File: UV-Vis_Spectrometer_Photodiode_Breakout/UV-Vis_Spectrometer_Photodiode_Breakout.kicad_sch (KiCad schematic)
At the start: 32 parts, among them J1 Conn_01x05, J2 Conn_01x02, J3 Conn_01x02, Q1 NMOS, Q2 NMOS, Q3 NMOS, U1 TLV8811DBVR, U3 LTC2451

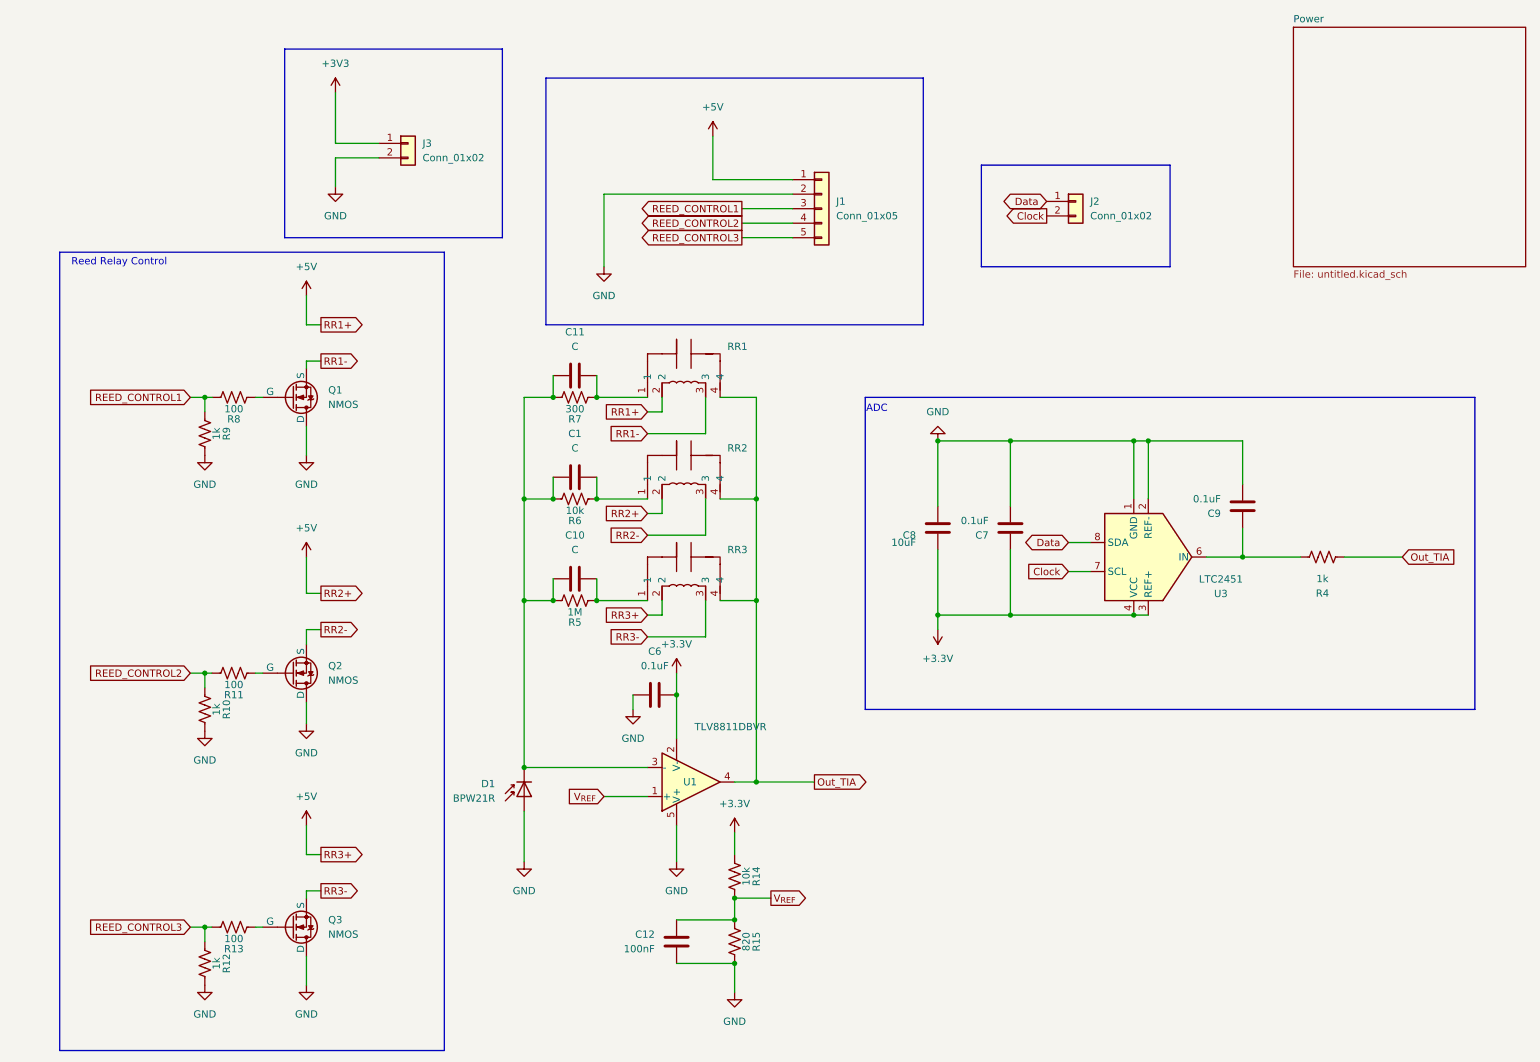
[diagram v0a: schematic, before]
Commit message: Made some nice boxes and labels.
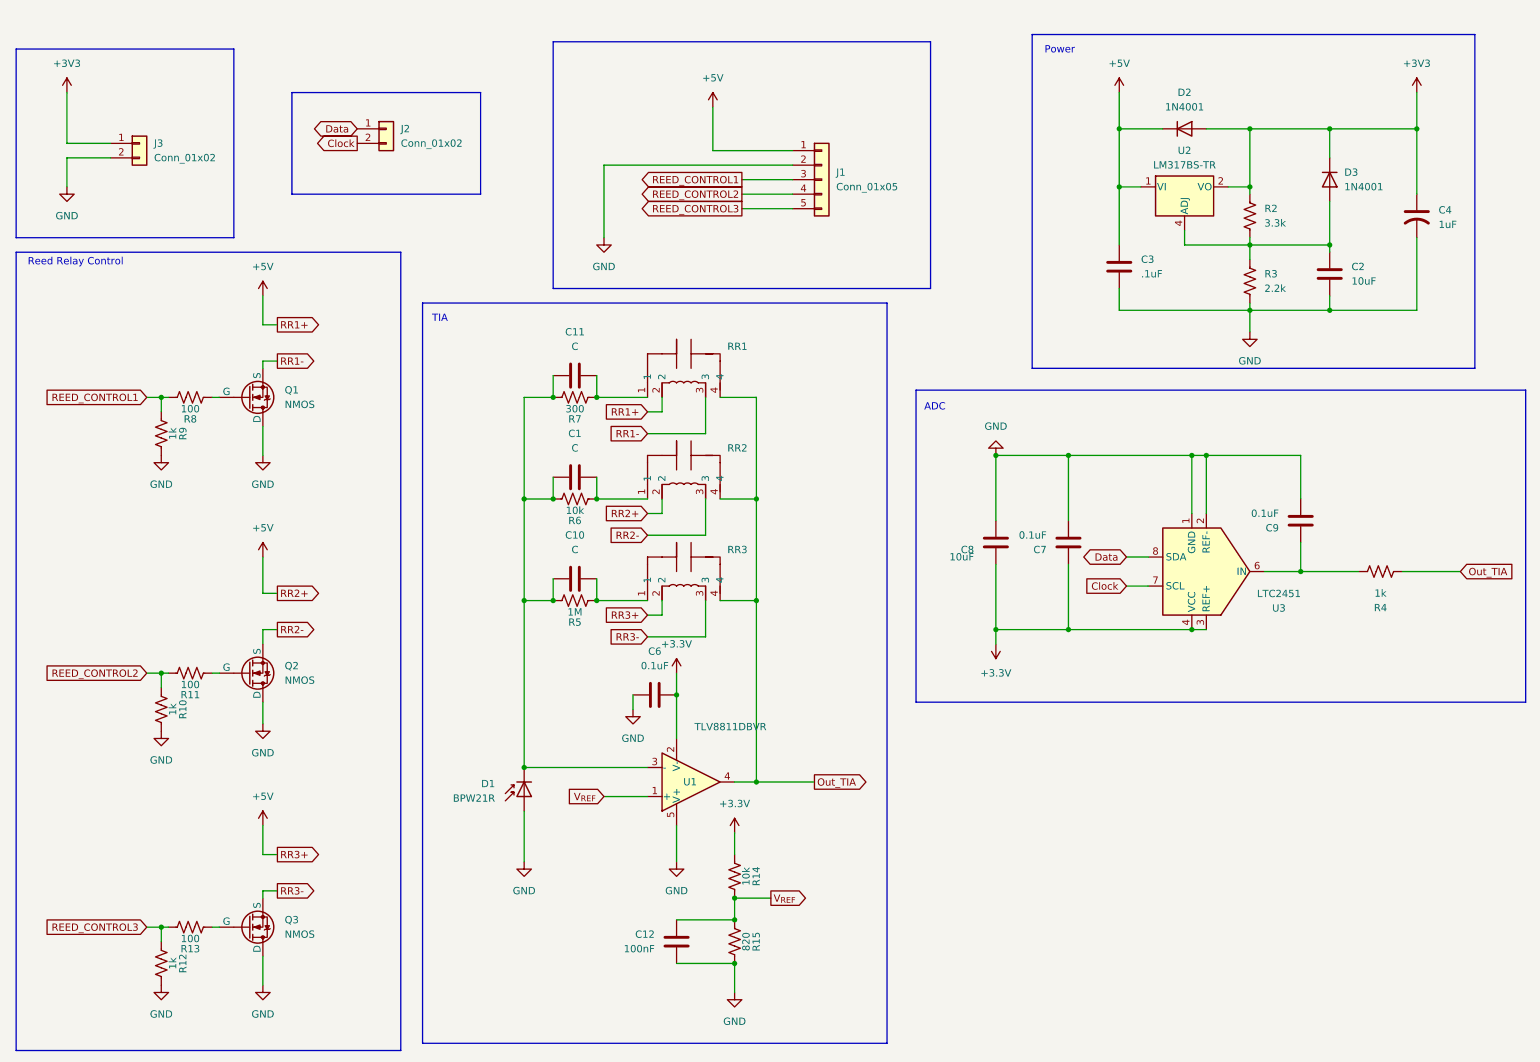
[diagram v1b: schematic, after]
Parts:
- added C2: 10uF, symbol Device:C
- added C3: .1uF, symbol Device:C
- added C4: 1uF, Package_SO:SOIC-8_3.9x4.9mm_P1.27mm, symbol Device:C_US
- added D2, D3: 1N4001, Diode_THT:D_DO-41_SOD81_P10.16mm_Horizontal, symbol Diode:1N4001
- added R2: 3.3k, Package_DIP:DIP-8_W7.62mm, symbol Device:R_US
- added R3: 2.2k, Package_DIP:DIP-8_W7.62mm, symbol Device:R_US
- added U2: LM317BS-TR, Package_SO:SOIC-8_3.9x4.9mm_P1.27mm, symbol Regulator_Linear:LM317L_SO8
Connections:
- net +3V3: now also C4.1, D2.2 (A), D3.1 (K), R2.1, U2.2 (VO), U2.3 (VO), U2.6 (VO), U2.7 (VO)
- net +5V: now also C3.1, D2.1 (K), U2.1 (VI)
- net GND: now also C2.2, C3.2, C4.2, R3.2
- new net: C2.1, D3.2 (A), R2.2, R3.1, U2.4 (ADJ)
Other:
- removed sheet Power
- note added: "Power"
- note added: "TIA"
- moved on the sheet: C7, C8, C9, J1, J2, J3, Q1, Q2, Q3, R10, R11, R12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
